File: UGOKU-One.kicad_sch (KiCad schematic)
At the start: 80 parts, among them J1 ENC/IO, J10 Conn_01x02, J12 Conn_01x02, J2 SERVO, J3 Conn_02x03_Odd_Even, J4 14110213001000, J5 Conn_01x05, J6 Conn_01x02, J7 ENC/IO, J8 DAC, J9 ADC, P1 USB_C_Plug_USB2.0, Q1 NMOS, Q2 SS8050, Q3 SS8050, SW2 SW_SPDT, SW3 SW_Slide_DPDT, SW4 SW_Push, SW5 SW_Slide_DPDT, SW6 SW_Push, U1 AMS1117-3.3, U2 CP2102N-A02-GQFN28, U3 TB67H450FNG_EL, U4 K7805M/M78AR05, U5 ESP32-WROOM-32E, U6 BMM150, U7 BMI270, U8 TB67H450FNG_EL

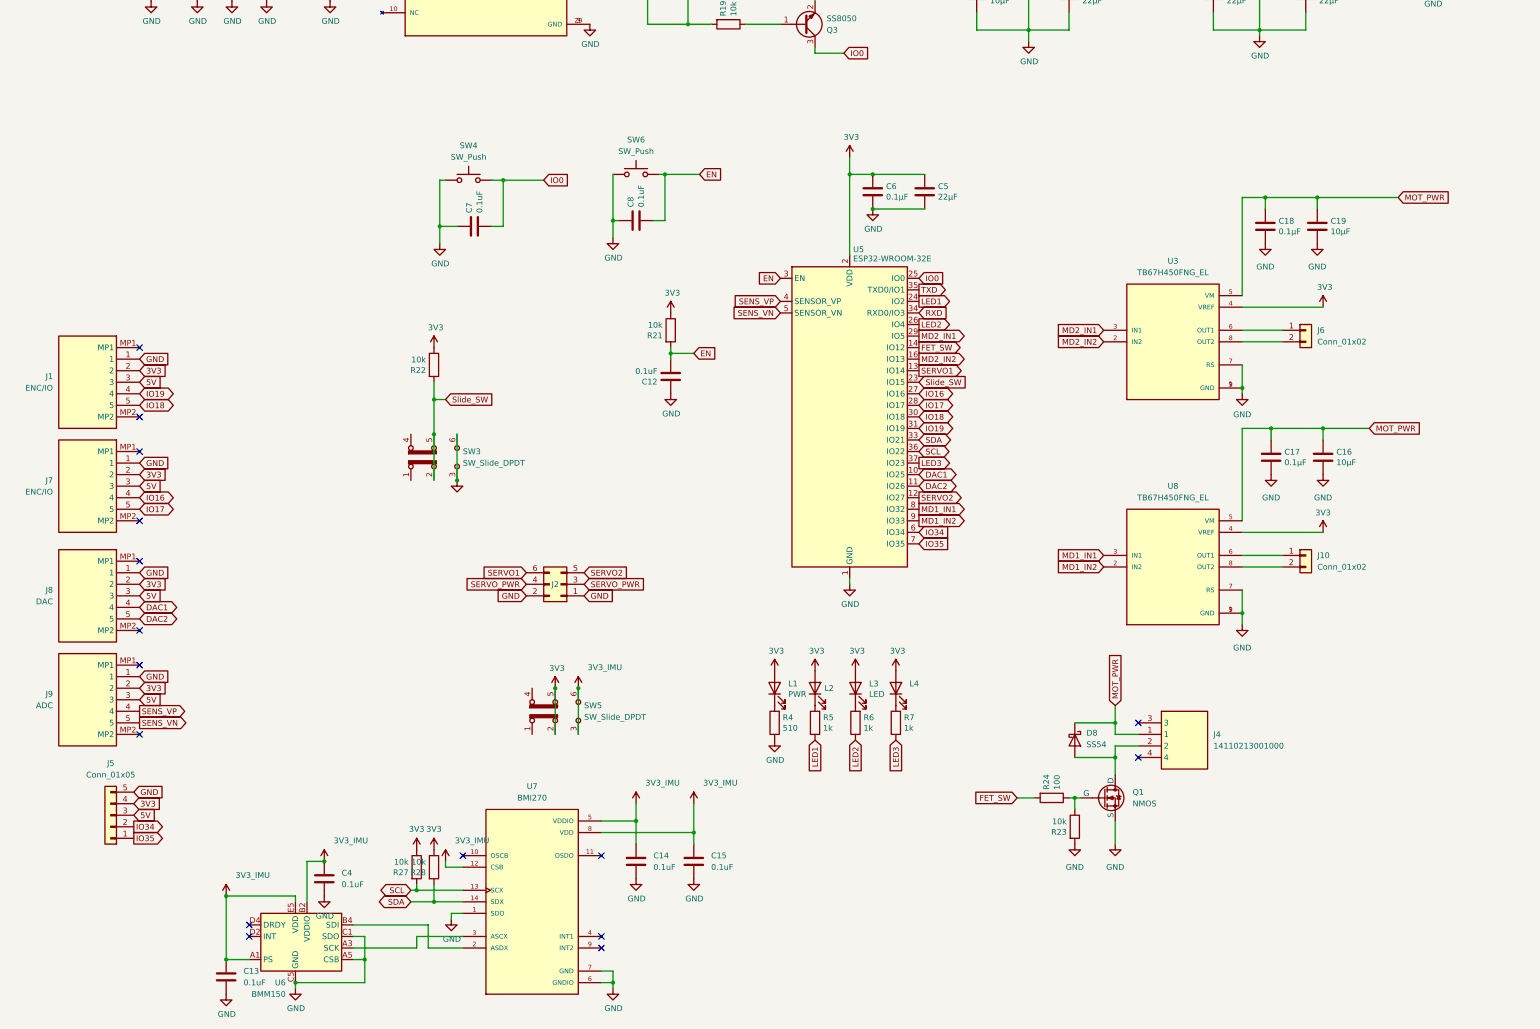
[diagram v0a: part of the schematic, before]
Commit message: April-22 order spec
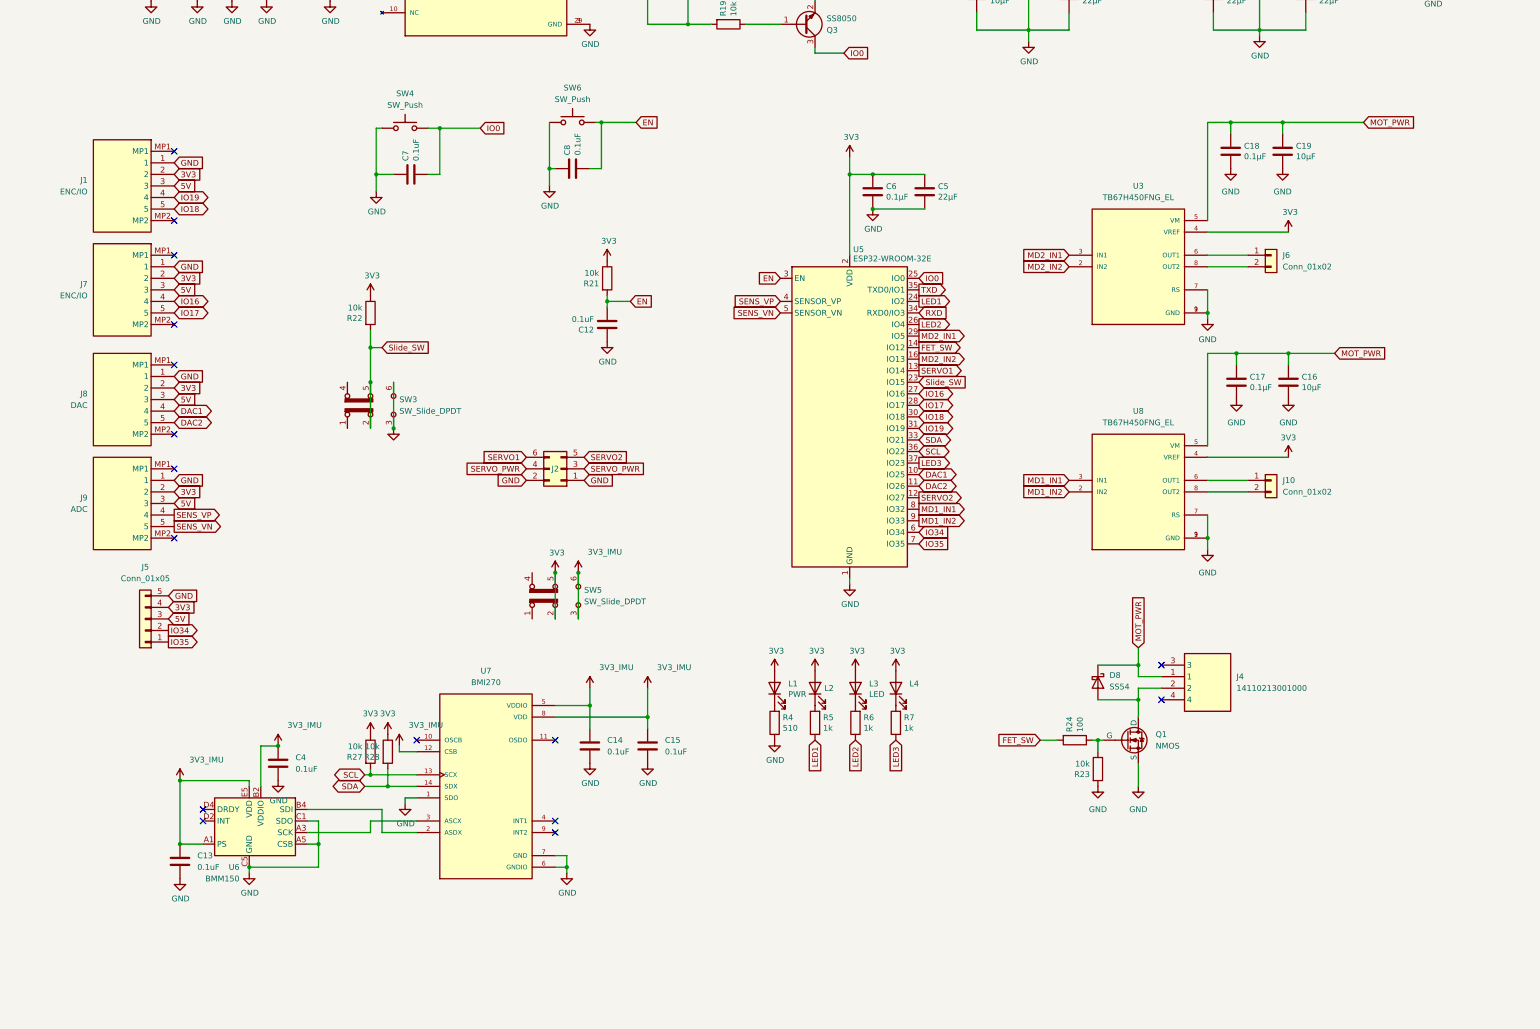
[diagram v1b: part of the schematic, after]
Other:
- moved on the sheet: C12, C13, C14, C15, C16, C17, C18, C19, C4, C7, C8, D8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
